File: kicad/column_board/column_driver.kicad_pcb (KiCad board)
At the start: 2 copper layers, 100 x 100 mm, 104 parts, among them J1 Panel column connector (femal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, J2 PWR_CHAIN_IN, J3 PWR_CHAIN_OUT, J4 DATA_CHAIN_IN, J5 DATA_CHAIN_OUT, U1 TPIC6B595, U10 TPIC6B595, U11 TPIC6B595, U12 TBD62783, U2 TPIC6B595, U3 TBD62783, U4 TPIC6B595, U5 TPIC6B595, U6 TBD62783, U7 TPIC6B595, U8 TPIC6B595, U9 TBD62783

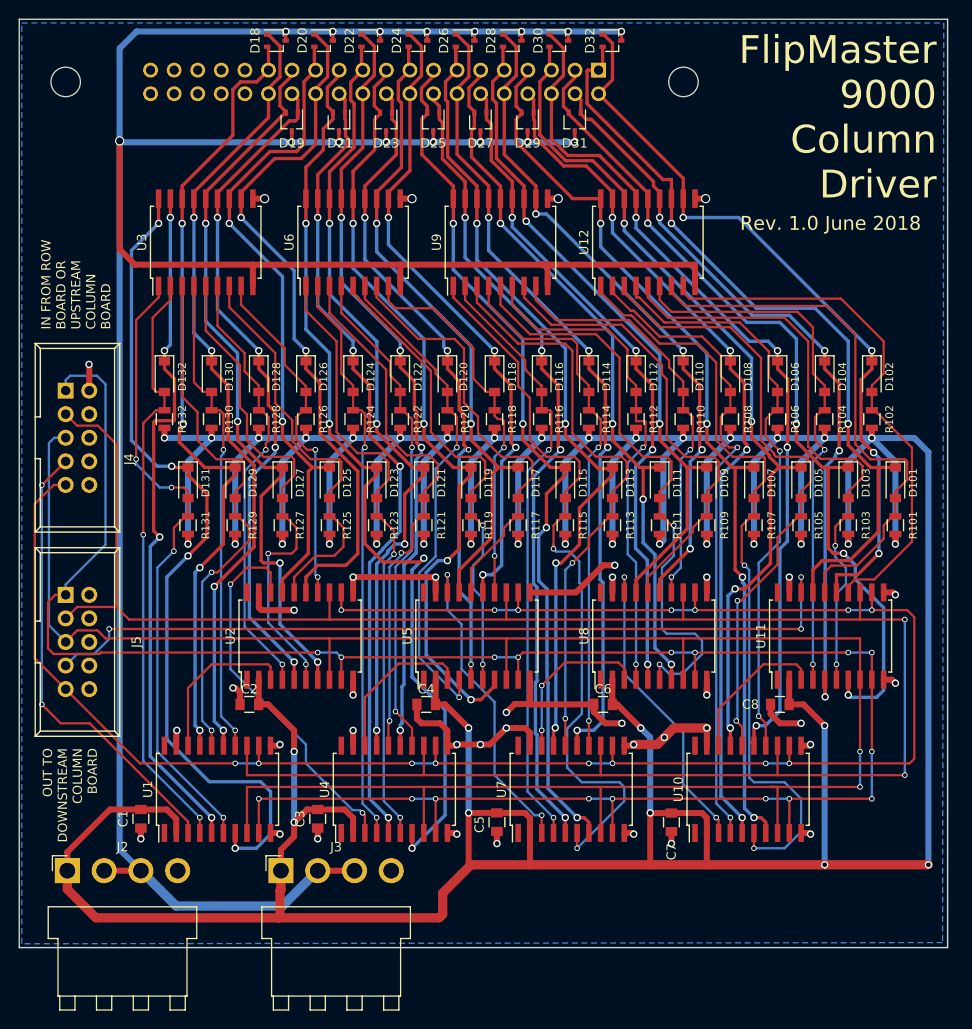
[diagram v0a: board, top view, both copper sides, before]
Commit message: Parts positioned
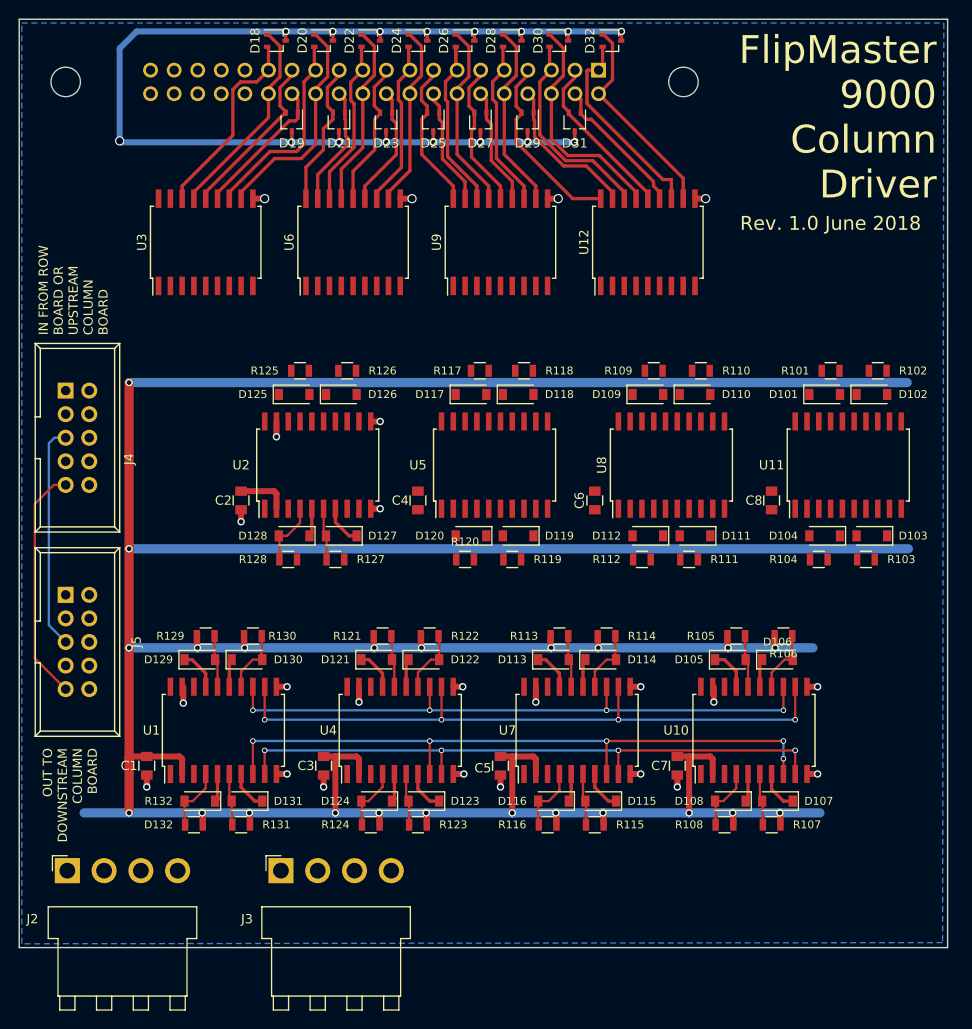
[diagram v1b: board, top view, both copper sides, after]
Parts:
- moved D132 45.9 mm to (44.5, 109.2), turned to 180 degrees
- moved D124 45.8 mm to (63.5, 109.2), turned to 180 degrees
- moved D116 45.7 mm to (82.5, 109.2), turned to 180 degrees
- moved D108 45.7 mm to (101.6, 109.2), turned to 180 degrees
- moved R132 43.8 mm to (43.8, 111.8), turned to 180 degrees
- moved R124 43.7 mm to (62.9, 111.8), turned to 180 degrees
- moved R108 43.7 mm to (101.0, 111.8), turned to 180 degrees
- moved R116 43.7 mm to (81.9, 111.8), turned to 180 degrees
- moved D131 34.9 mm to (49.5, 109.2), turned to 180 degrees
- moved D123 34.7 mm to (68.6, 109.2), turned to 180 degrees
- moved D115 34.5 mm to (87.6, 109.2), turned to 180 degrees
- moved D107 34.4 mm to (106.7, 109.2), turned to 180 degrees
- moved R131 32.8 mm to (48.9, 111.8), turned to 180 degrees
- moved R123 32.6 mm to (67.9, 111.8), turned to 180 degrees
- moved R115 32.4 mm to (87.0, 111.8), turned to 180 degrees
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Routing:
- net +24V: track 323.9 -> 130.1 mm
- net +5V: track 606.2 -> 435.6 mm, vias 41 -> 23
- net ~COL_EN: track 231.4 -> 67.5 mm, vias 17 -> 4
- net RC_SHIFT_CLK: track 227.8 -> 67.5 mm, vias 2 -> 4
- net ~RC_CLEAR: track 226.6 -> 95.8 mm, vias 2 -> 5
- net COL_REG_CLK: track 213.0 -> 97.1 mm, vias 15 -> 4
- net RC_DATA_OUT: track 88.7 -> 0.00 mm, vias 3 -> 0
- net COL31: track 90.6 -> 4.34 mm, vias 4 -> 0
- net GND: track 116.0 -> 30.0 mm, vias 38 -> 24
- net COL23: track 101.2 -> 20.3 mm, vias 4 -> 0
- net Net-(D107-Pad2): track 84.2 -> 5.59 mm, vias 2 -> 0
- net Net-(D115-Pad2): track 81.5 -> 5.59 mm, vias 2 -> 0
- net COL3: track 92.7 -> 18.1 mm, vias 4 -> 0
- net COL7: track 98.8 -> 24.8 mm, vias 4 -> 0
- net COL15: track 94.4 -> 20.6 mm, vias 4 -> 0
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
